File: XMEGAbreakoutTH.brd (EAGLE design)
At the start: 160 x 100 mm, 23 parts, among them IC1 XMEGA16A4

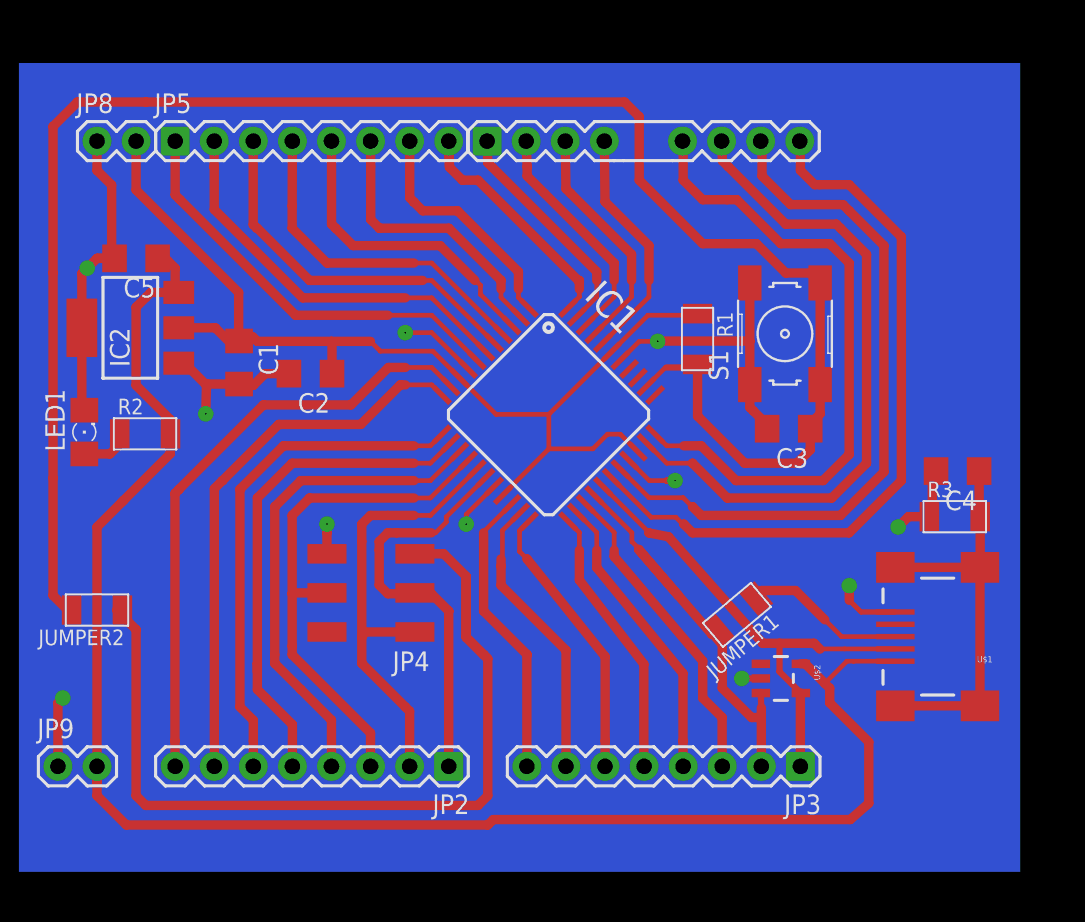
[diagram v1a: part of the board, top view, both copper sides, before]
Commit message: latest
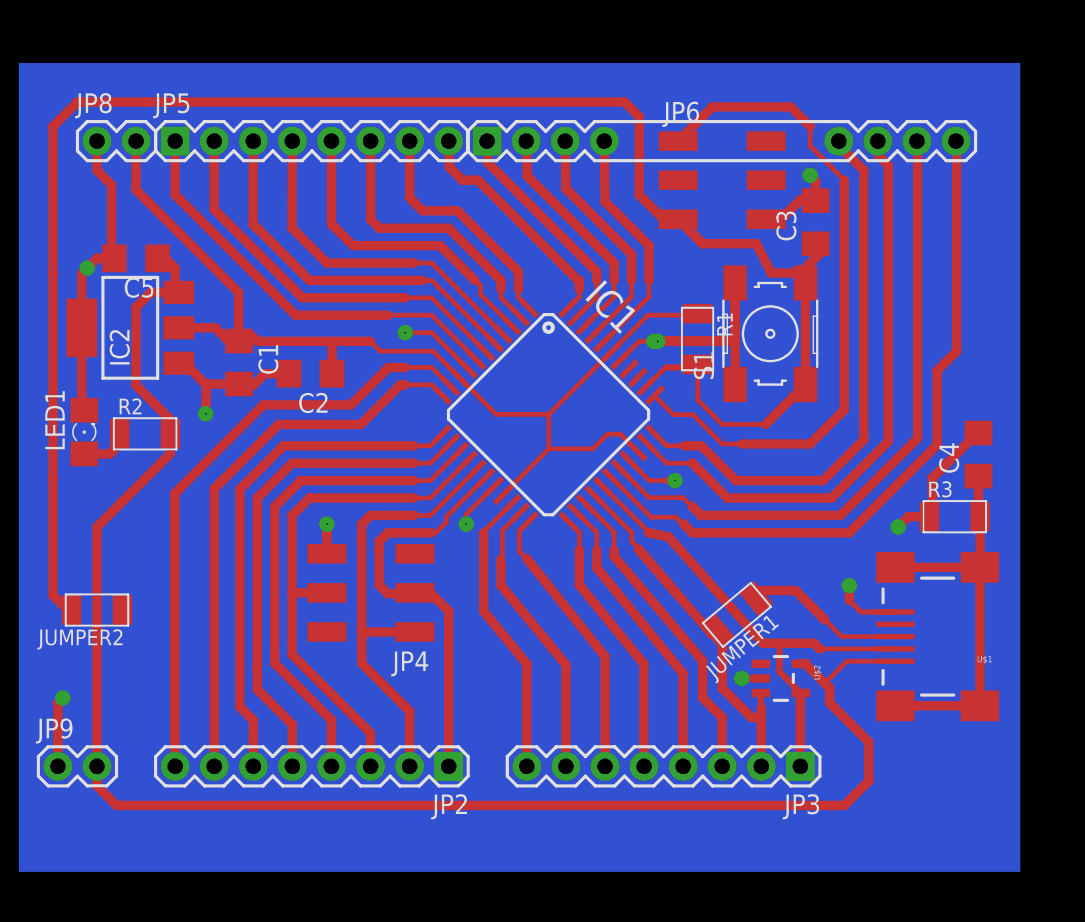
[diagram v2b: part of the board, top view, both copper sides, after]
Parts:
- added JP6: (no value), fab:2X03SMD
- moved C3 13.5 mm to (91.2, 57.0), turned to 90 degrees
- moved C4 1.73 mm to (101.7, 41.9), turned to 90 degrees
- moved S1 0.95 mm to (88.2, 49.7)
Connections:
- new net DAT: IC1.34, JP6.1
- net GND: now also JP6.6
- net RESET: now also JP6.5; no longer JP4.5
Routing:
- net RESET: track 177.6 -> 116.3 mm
- net DAT: track 0.00 -> 43.9 mm
- net GND: track 218.0 -> 246.9 mm, vias 11 -> 12
- net PE3: track 42.6 -> 36.0 mm
- net PE2: track 43.5 -> 38.5 mm
- net PE1: track 46.4 -> 42.0 mm
- net PE0: track 47.8 -> 45.3 mm
- net VBUS: track 110.6 -> 108.3 mm
